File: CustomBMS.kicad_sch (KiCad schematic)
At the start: 0 parts

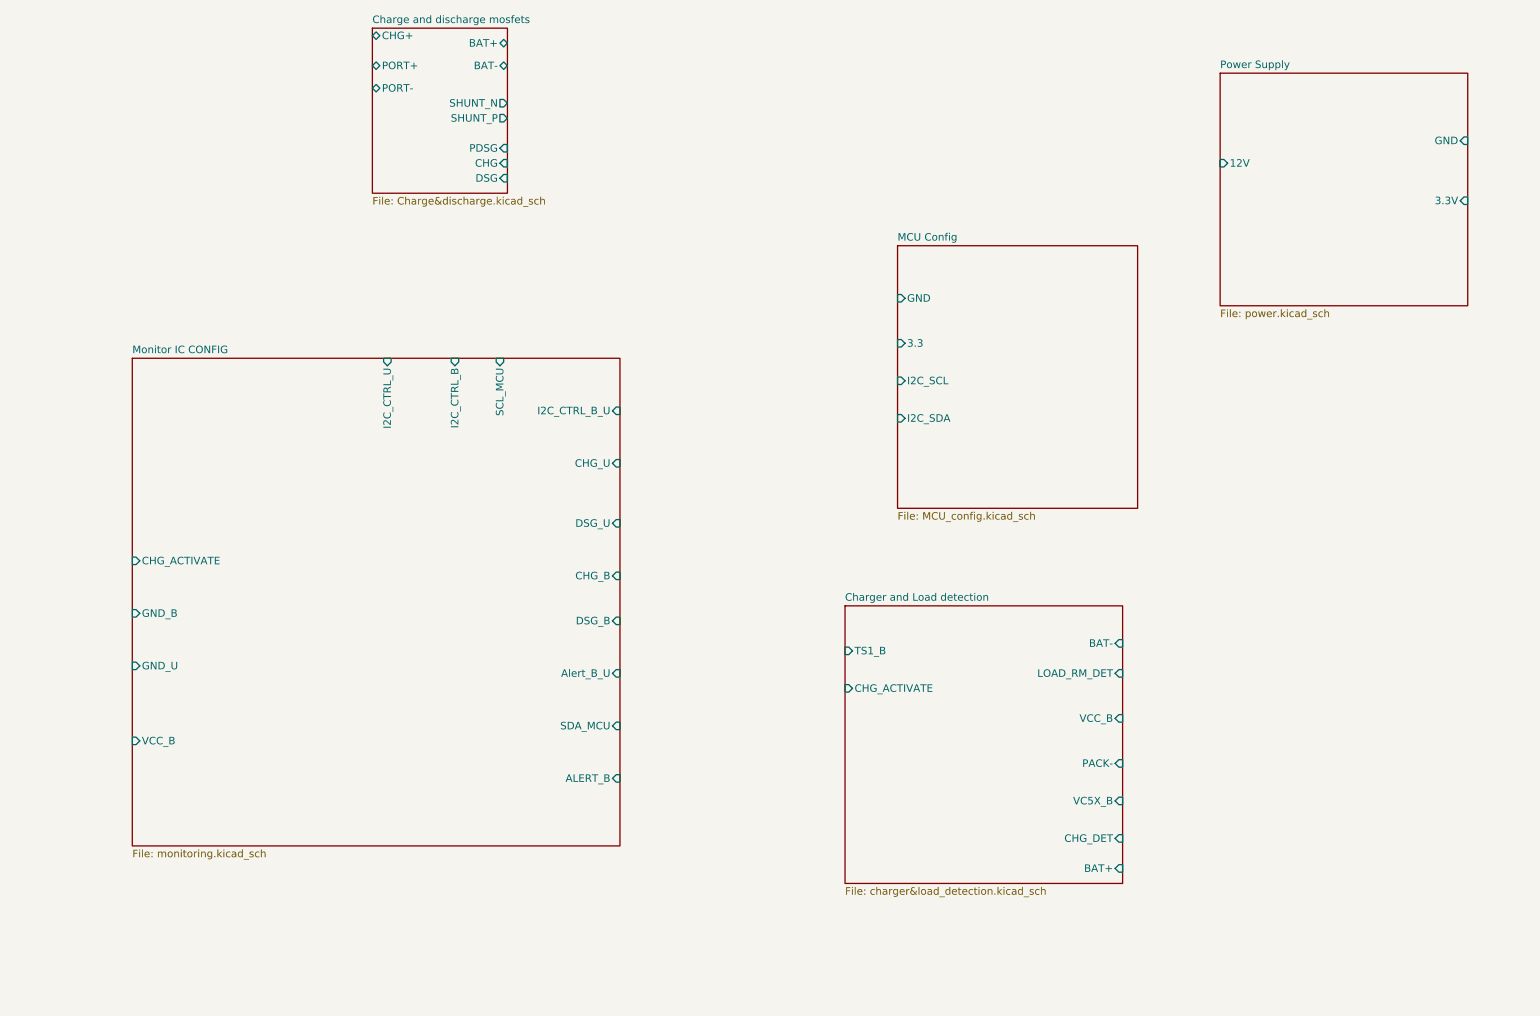
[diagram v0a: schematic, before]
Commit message: schematic v0
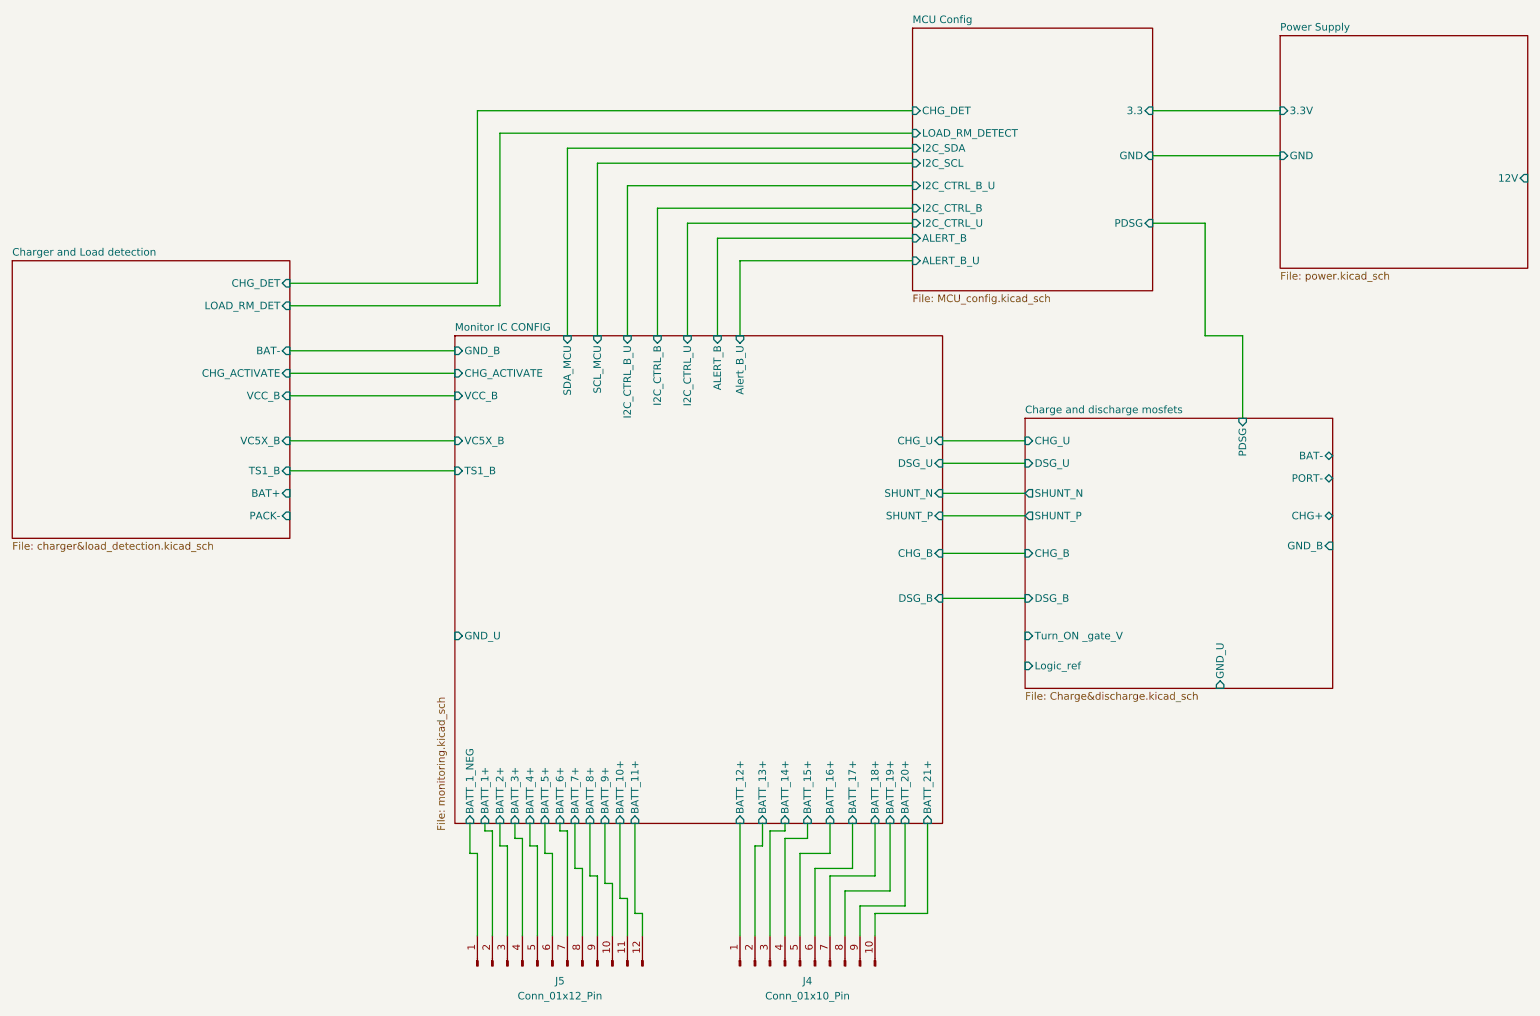
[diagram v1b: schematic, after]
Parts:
- added J4: Conn_01x10_Pin, symbol Connector:Conn_01x10_Pin
- added J5: Conn_01x12_Pin, symbol Connector:Conn_01x12_Pin
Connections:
- new net Monitor IC CONFIG/BATT_1+: J5.2 (Pin_2)
- new net Monitor IC CONFIG/BATT_10+: J5.11 (Pin_11)
- new net Monitor IC CONFIG/BATT_11+: J5.12 (Pin_12)
- new net Monitor IC CONFIG/BATT_12+: J4.1 (Pin_1)
- new net Monitor IC CONFIG/BATT_13+: J4.2 (Pin_2)
- new net Monitor IC CONFIG/BATT_14+: J4.3 (Pin_3)
- new net Monitor IC CONFIG/BATT_15+: J4.4 (Pin_4)
- new net Monitor IC CONFIG/BATT_16+: J4.5 (Pin_5)
- new net Monitor IC CONFIG/BATT_17+: J4.6 (Pin_6)
- new net Monitor IC CONFIG/BATT_18+: J4.7 (Pin_7)
- new net Monitor IC CONFIG/BATT_19+: J4.8 (Pin_8)
- new net Monitor IC CONFIG/BATT_1_NEG: J5.1 (Pin_1)
- new net Monitor IC CONFIG/BATT_2+: J5.3 (Pin_3)
- new net Monitor IC CONFIG/BATT_20+: J4.9 (Pin_9)
- new net Monitor IC CONFIG/BATT_21+: J4.10 (Pin_10)
- new net Monitor IC CONFIG/BATT_3+: J5.4 (Pin_4)
- new net Monitor IC CONFIG/BATT_4+: J5.5 (Pin_5)
- new net Monitor IC CONFIG/BATT_5+: J5.6 (Pin_6)
- new net Monitor IC CONFIG/BATT_6+: J5.7 (Pin_7)
- new net Monitor IC CONFIG/BATT_7+: J5.8 (Pin_8)
- new net Monitor IC CONFIG/BATT_8+: J5.9 (Pin_9)
- new net Monitor IC CONFIG/BATT_9+: J5.10 (Pin_10)
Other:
- sheet Charge and discharge mosfets ports: added CHG_B, CHG_U, DSG_B, DSG_U, GND_B, GND_U, Logic_ref, Turn_ON _gate_V; removed BAT+, CHG, DSG, PORT+
- sheet MCU Config ports: added ALERT_B, ALERT_B_U, CHG_DET, I2C_CTRL_B, I2C_CTRL_B_U, I2C_CTRL_U, LOAD_RM_DETECT, PDSG; removed none
- sheet Monitor IC CONFIG ports: added BATT_1+, BATT_10+, BATT_11+, BATT_12+, BATT_13+, BATT_14+, BATT_15+, BATT_16+, BATT_17+, BATT_18+, BATT_19+, BATT_1_NEG, BATT_2+, BATT_20+, BATT_21+, BATT_3+, BATT_4+, BATT_5+, BATT_6+, BATT_7+, BATT_8+, BATT_9+, SHUNT_N, SHUNT_P, TS1_B, VC5X_B; removed none
